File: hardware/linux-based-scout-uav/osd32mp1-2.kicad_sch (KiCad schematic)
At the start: 1 part, among them U1 OSD32MP157C-512M-IAA

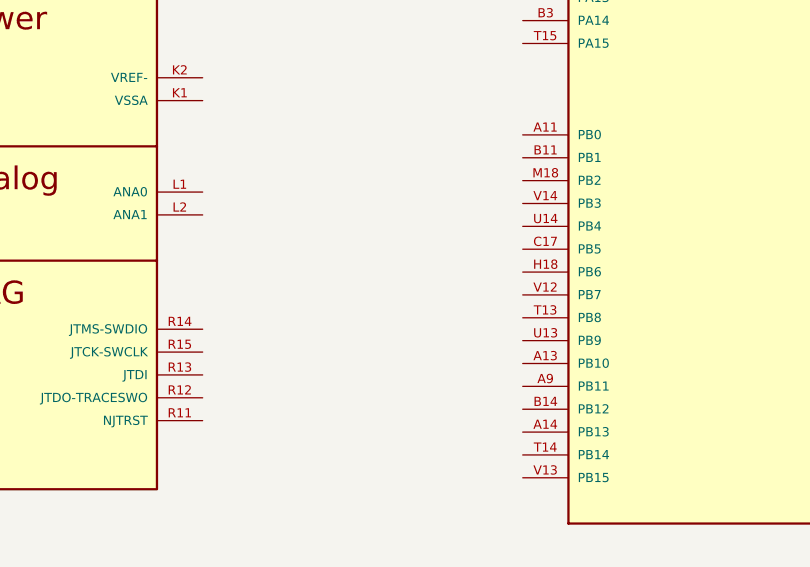
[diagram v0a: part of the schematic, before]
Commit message: Schematic update
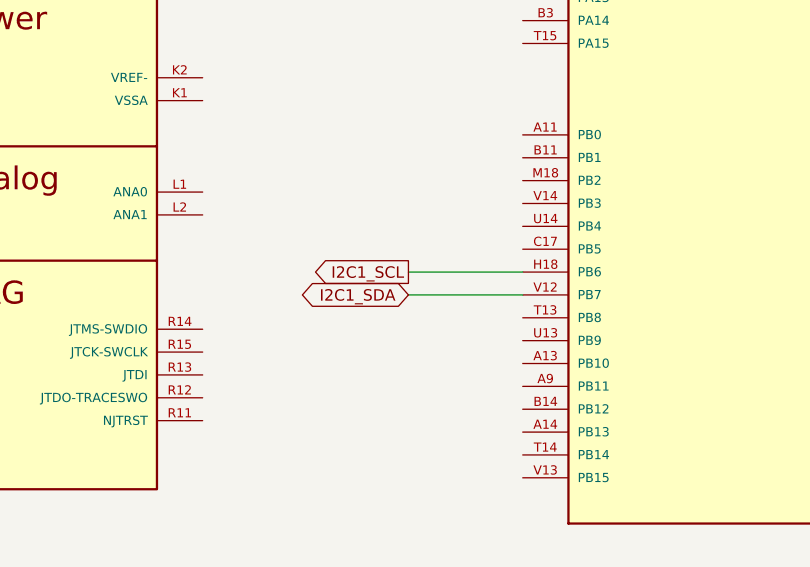
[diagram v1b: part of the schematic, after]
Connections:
- net I2C1_SCL: now reaches U1.H18 (PB6)
- net I2C1_SDA: now reaches U1.V12 (PB7)
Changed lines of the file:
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@@
+	(wire
+		(pts
+			(xy 177.8 147.32) (xy 190.5 147.32)
+		)
+		(stroke
+			(width 0)
+			(type default)
+		)
+	)
+	(wire
+		(pts
+			(xy 177.8 149.86) (xy 190.5 149.86)
+		)
+		(stroke
+			(width 0)
+			(type default)
+		)
+	)
 	(wire
 		(pts
@@
 				(hide yes)
 			)
+		)
+	)
+	(global_label "I2C1_SCL"
+		(shape output)
+		(at 177.8 147.32 180)
+		(fields_autoplaced yes)
+		(effects
+			(font
+				(size 1.27 1.27)
+			)
+			(justify right)
+		)
+		(property "Intersheetrefs" "${INTERSHEET_REFS}"
+			(at 166.0458 147.32 0)
+			(effects
+				(font
+					(size 1.27 1.27)
+				)
+				(justify right)
+				(hide yes)
+			)
+		)
+	)
+	(global_label "I2C1_SDA"
+		(shape bidirectional)
+		(at 177.8 149.86 180)
+		(fields_autoplaced yes)
+		(effects
+			(font
+				(size 1.27 1.27)
+			)
+			(justify right)
+		)
+		(property "Intersheetrefs" "${INTERSHEET_REFS}"
+			(at 164.874 149.86 0)
+			(effects
+				(font
+					(size 1.27 1.27)
+				)
+				(justify right)
+				(hide yes)
+			)

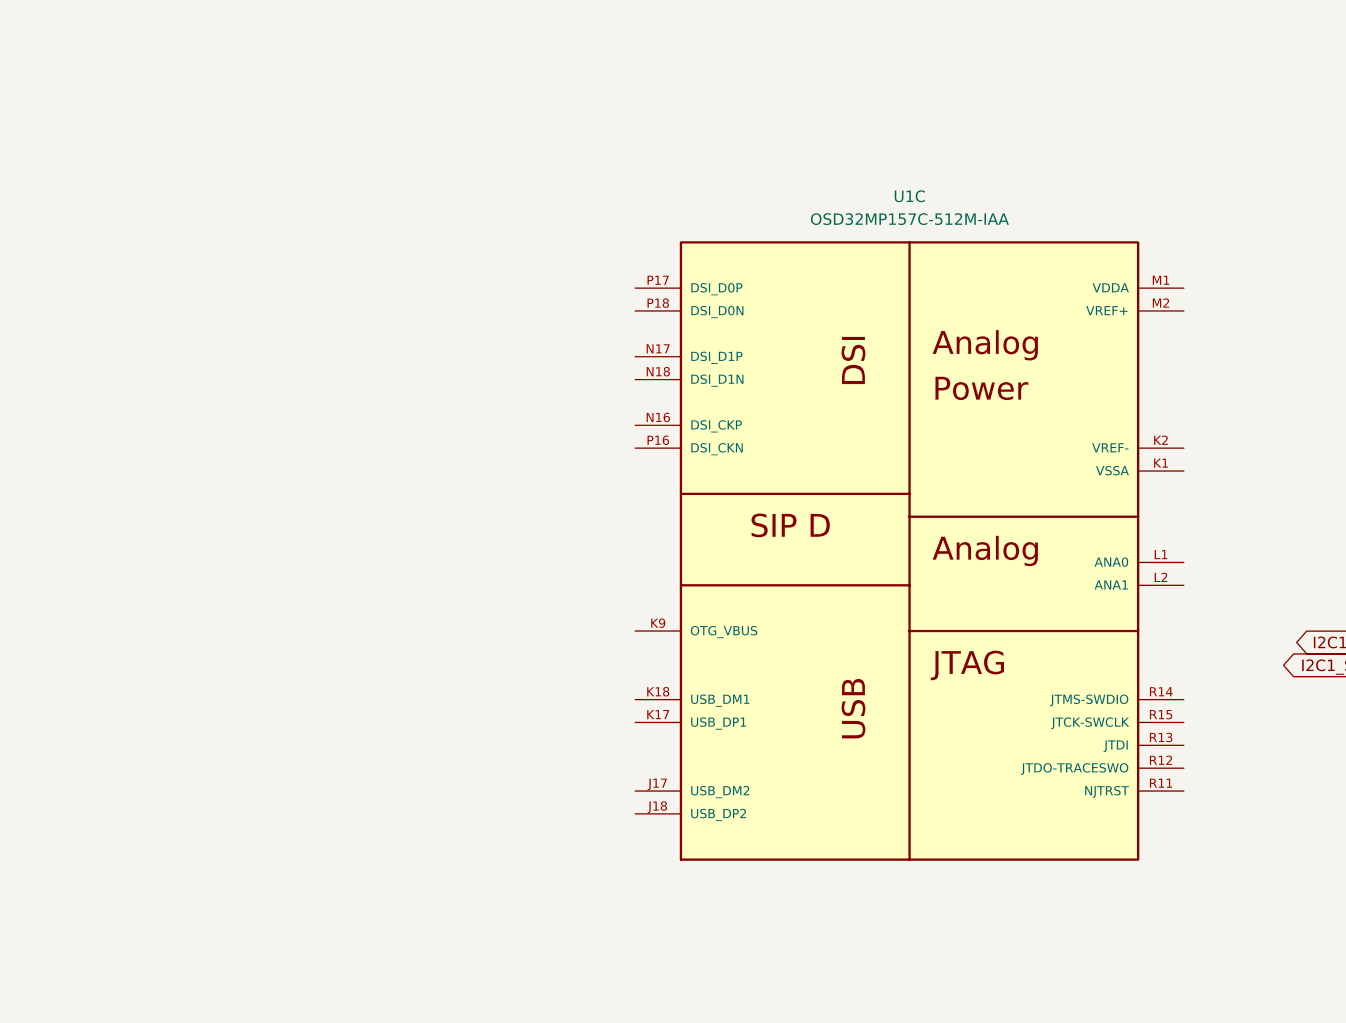
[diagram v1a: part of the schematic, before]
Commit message: Schematic update
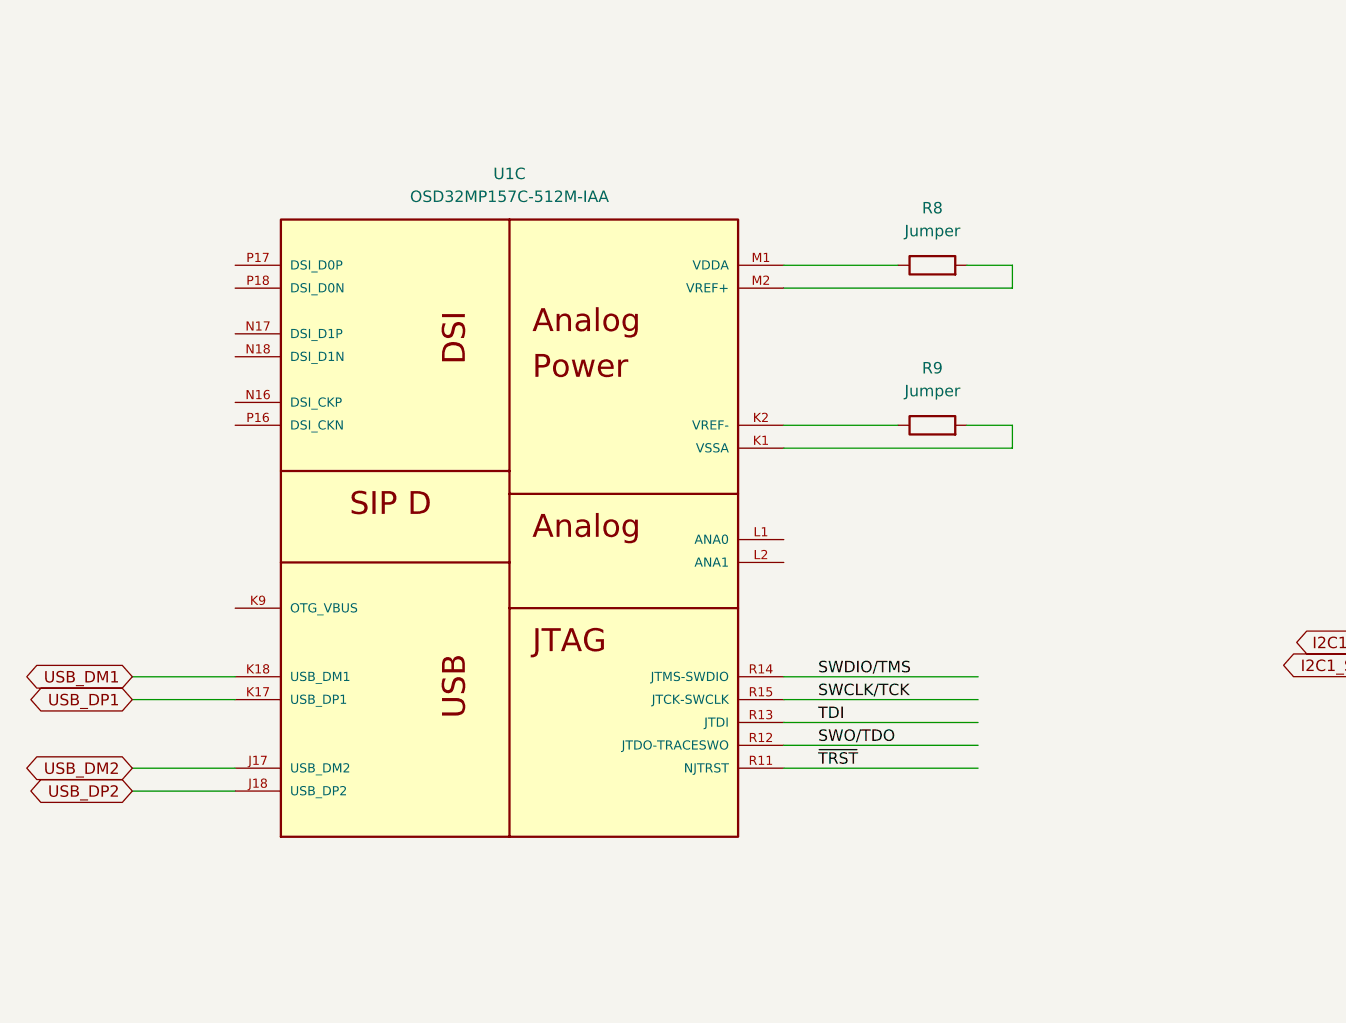
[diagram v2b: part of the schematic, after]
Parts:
- added R8, R9: Jumper, Resistor_SMD:R_0402_1005Metric, symbol Device:R
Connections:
- net USB_DM2: now reaches U1.J17 (USB_DM2)
- net USB_DP2: now reaches U1.J18 (USB_DP2)
- net at U1.K1 (VSSA): now also R9.2
- net USB_DP1: now reaches U1.K17 (USB_DP1)
- net USB_DM1: now reaches U1.K18 (USB_DM1)
- net at U1.K2 (VREF-): now also R9.1
- net at U1.M1 (VDDA): now also R8.1
- net at U1.M2 (VREF+): now also R8.2
- net ~{TRST}: now reaches U1.R11 (NJTRST)
- net SWO/TDO: now reaches U1.R12 (JTDO-TRACESWO)
- net TDI: now reaches U1.R13 (JTDI)
- net SWDIO/TMS: now reaches U1.R14 (JTMS-SWDIO)
- net SWCLK/TCK: now reaches U1.R15 (JTCK-SWCLK)
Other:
- moved on the sheet: U1C
